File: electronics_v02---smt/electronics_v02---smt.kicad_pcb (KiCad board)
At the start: 4 copper layers, 26.7 x 92.7 mm, 24 parts, among them IC1 SN74HCT245PWR, IC2 MAX3485EESA+T, J1 171857-0004, J2 171857-0004, J3 171857-0003, J4 171857-0002, U1 RPiPicoW

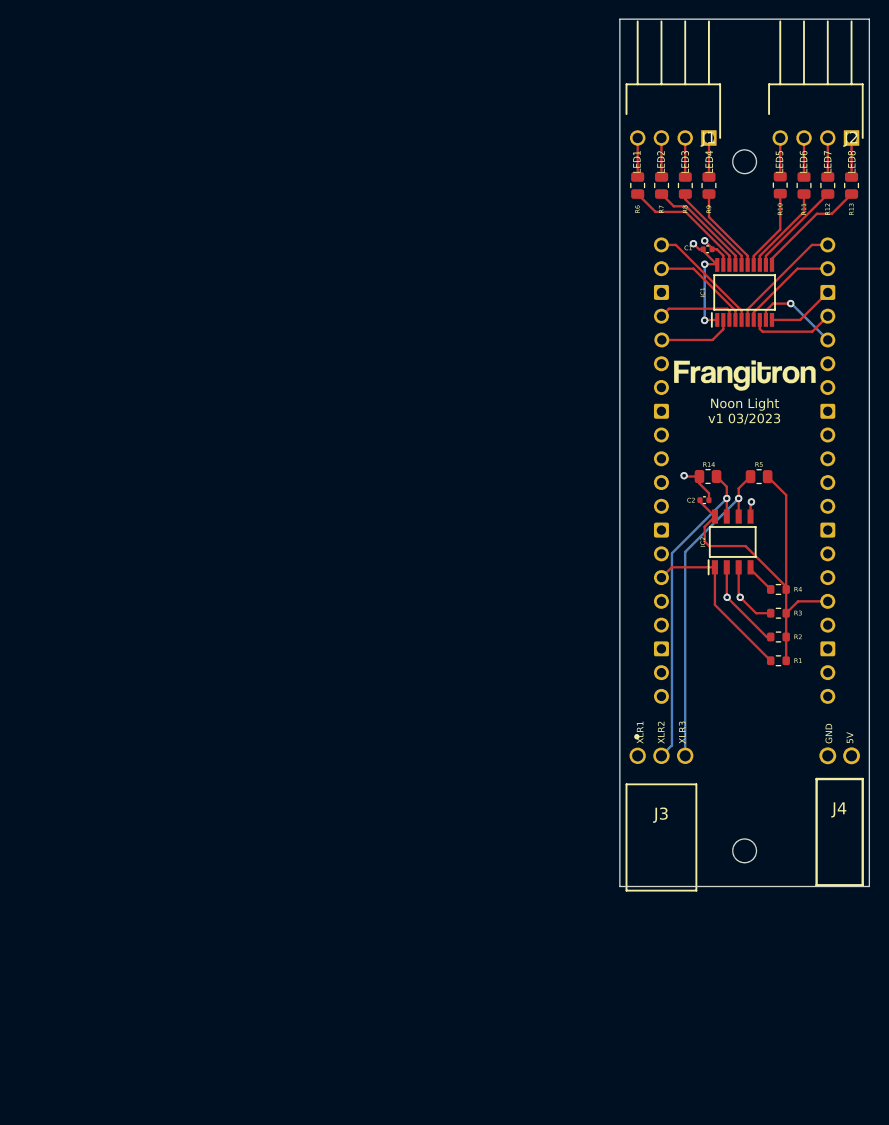
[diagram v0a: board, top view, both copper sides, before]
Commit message: Add files via upload
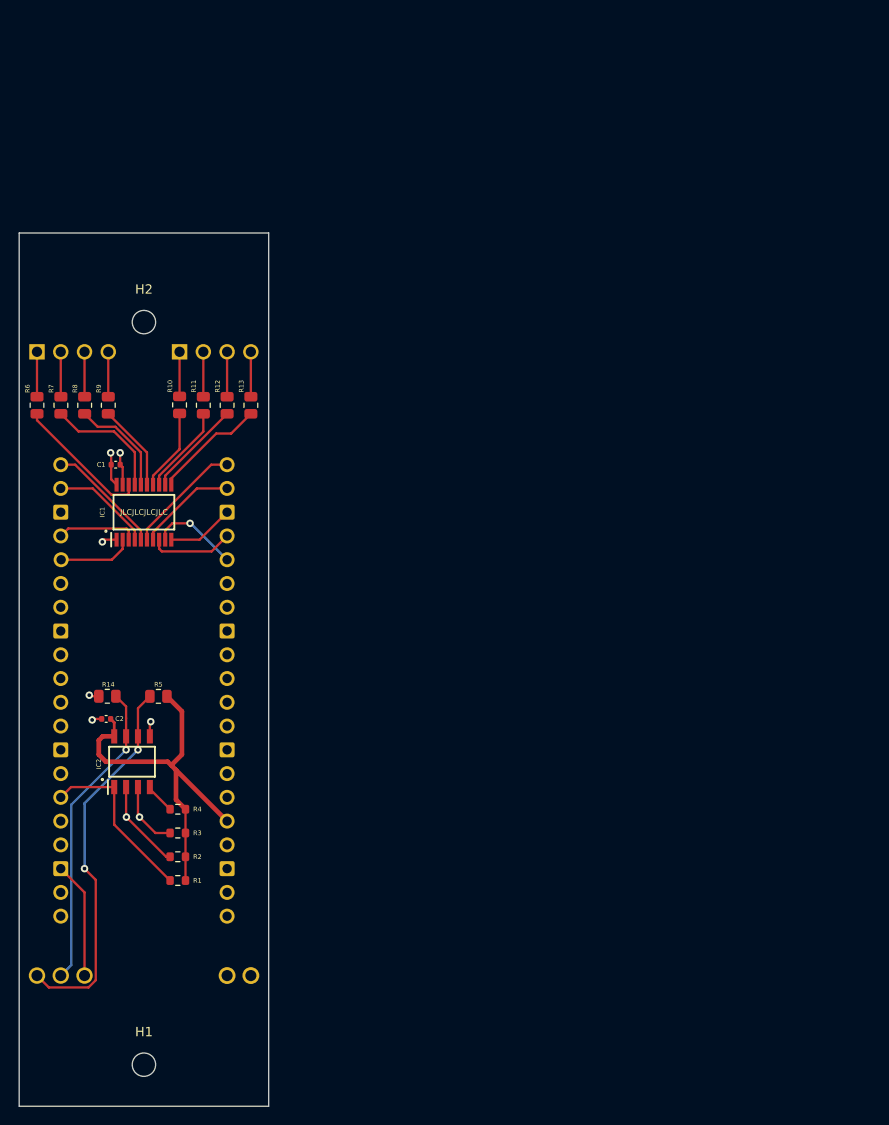
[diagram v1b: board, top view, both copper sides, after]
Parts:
- added H1: MountingHole, MountingHole:MountingHole_2.5mm, F.Cu at (140.3, 137.2)
- added H2: MountingHole, MountingHole:MountingHole_2.5mm, F.Cu at (140.3, 57.8)
- HS1, J1, J2, J3, J4: moved to B.Cu
- moved J2 75.4 mm to (144.1, 61.0), turned to 180 degrees
- moved J1 75.4 mm to (128.8, 61.0), turned to 180 degrees
- moved IC1 68.4 mm to (140.3, 78.1)
- moved J3 68.4 mm to (131.4, 133.9), turned to 0 degrees
- moved R1 68.4 mm to (143.9, 117.5)
- moved R10 68.4 mm to (144.1, 66.6)
- moved R12 68.4 mm to (149.2, 66.7)
- moved R13 68.4 mm to (151.7, 66.7)
- moved R14 68.4 mm to (136.3, 97.8)
- moved R2 68.4 mm to (143.9, 114.9)
- moved R3 68.4 mm to (143.9, 112.4)
- moved R4 68.4 mm to (143.9, 109.9)
- moved R5 68.4 mm to (141.8, 97.8)
- moved R7 68.4 mm to (131.4, 66.7)
- moved R9 68.4 mm to (136.5, 66.7)
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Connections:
- net XLR 1 renamed XLR1/GND
- J1 pad 1: LED_4 -> LED_1
- J1 pad 2: LED_3 -> LED_2
- J1 pad 3: LED_2 -> LED_3
- J1 pad 4: LED_1 -> LED_4
- J2 pad 1: LED_8 -> LED_5
- J2 pad 2: LED_7 -> LED_6
- J2 pad 3: LED_6 -> LED_7
- J2 pad 4: LED_5 -> LED_8
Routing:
- net XLR1/GND: track 34.0 -> 43.8 mm, vias 5 -> 6
- net +5V: track 12.3 -> 5.29 mm, vias 3 -> 2
- net XLR 3: track 34.7 -> 40.9 mm, vias 1 -> 2
- net XLR 2: track 35.1 -> 33.2 mm
- net Net-(IC1-Pad17): track 11.6 -> 13.1 mm
- net Net-(IC1-Pad18): track 13.5 -> 14.8 mm
- net Net-(IC1-Pad16): track 10.1 -> 11.2 mm
- net +3.3V: track 42.0 -> 42.8 mm
- net LED_3: track 4.17 -> 4.81 mm
- net LED_8: track 4.17 -> 4.80 mm
- net LED_7: track 4.17 -> 4.80 mm
- net LED_6: track 4.17 -> 4.80 mm
- net LED_5: track 4.13 -> 4.77 mm
- net LED_4: track 4.17 -> 4.80 mm
- net LED_2: track 4.17 -> 4.81 mm
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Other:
- board size 26.7 x 92.7 mm -> 26.7 x 93.3 mm
- board text added: "JLCJLCJLCJLC"
- board text added: "Noon Light v1 02/2023"
- board text removed: "Noon Light v1 03/2023"
